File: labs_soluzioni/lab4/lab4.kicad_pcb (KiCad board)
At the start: 6 copper layers, 100 x 100 mm, 1 part, among them U1 XC7A35T-FGG484

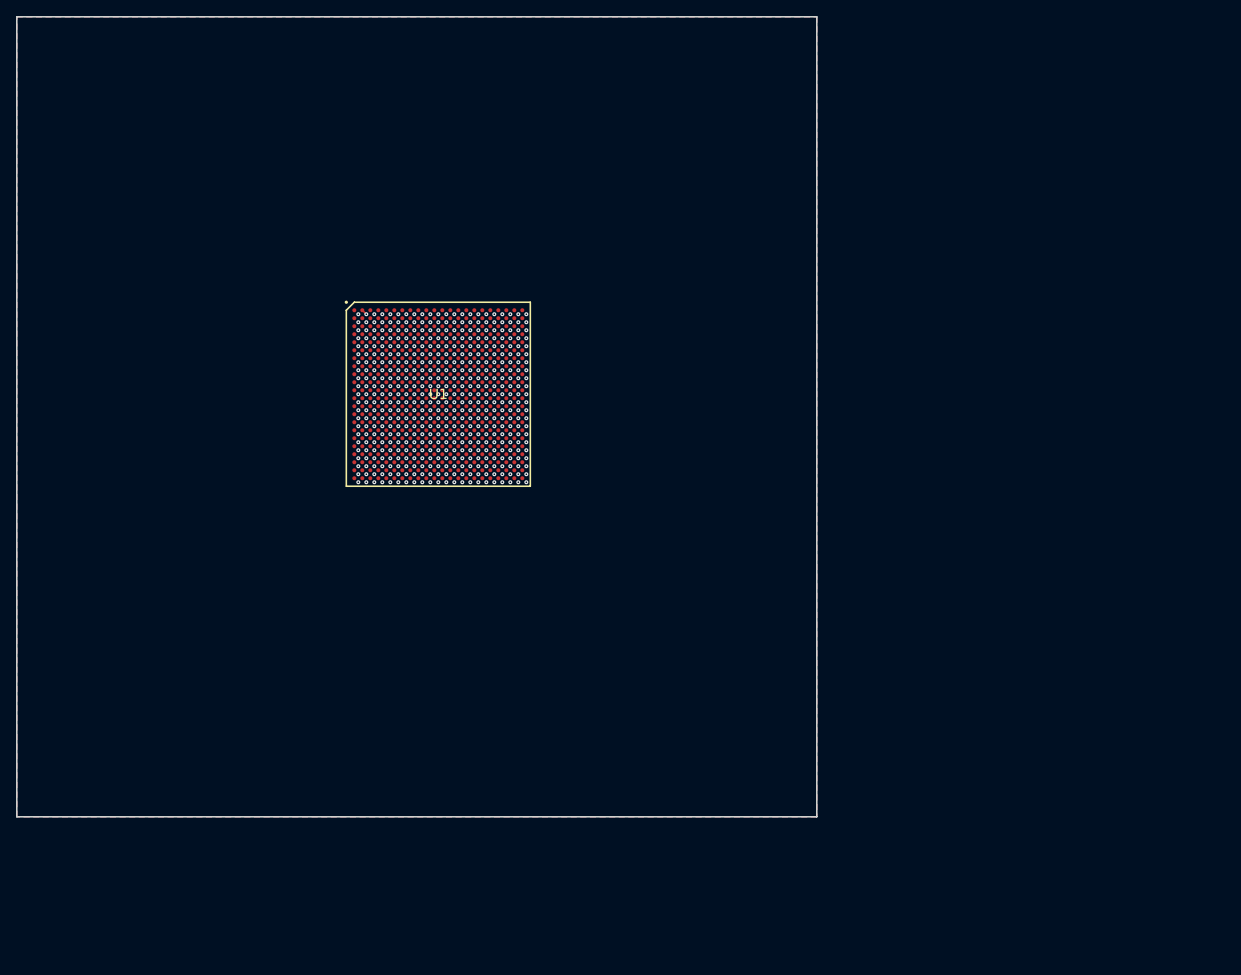
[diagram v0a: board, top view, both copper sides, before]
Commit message: NEW lab4
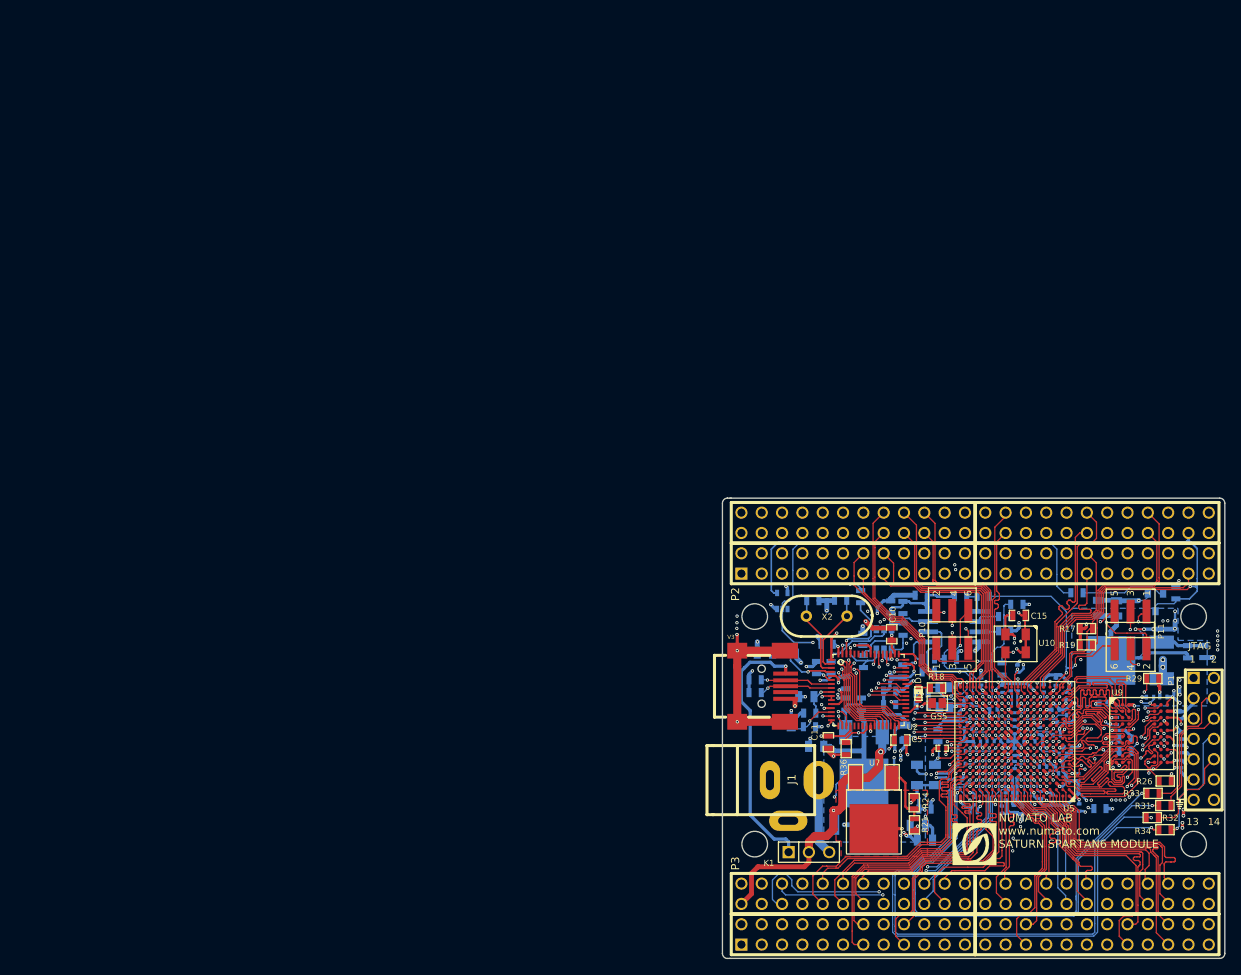
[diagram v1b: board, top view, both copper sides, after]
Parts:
- added 1PIN: P***, MH-3.2MM, F.Cu at (142.2, 125.0)
- added 1PIN: P***, MH-3.2MM, F.Cu at (197.1, 125.0)
- added 1PIN: P***, MH-3.2MM, F.Cu at (197.1, 153.4)
- added 1PIN: P***, MH-3.2MM, F.Cu at (142.2, 153.4)
- added C1: 0.1uF, SM0603_Capa, B.Cu at (151.3, 128.4)
- added C10: 0.1uF, SM0603_Capa, F.Cu at (159.4, 127.2)
- added C11: 0.1uF, SM0603_Capa, F.Cu at (151.5, 140.7)
- added C12: 0.1uF, SM0603_Capa, B.Cu at (155.8, 127.8)
- added C13: 0.1uF, SM0603_Capa, B.Cu at (146.7, 129.5)
- added C14: 0.1uF, SM0603_Capa, B.Cu at (149.1, 137.0)
- added C15: 0.1uF, SM0603_Capa, F.Cu at (175.3, 124.8)
- added C16: 15pF, SM0603_Capa, B.Cu at (165.1, 139.9)
- added C17: 0.01uF, SM0603_Capa, B.Cu at (159.1, 134.3)
- added C18: 0.01uF, SM0402_c, B.Cu at (177.9, 139.3)
- added C19: 0.01uF, SM0402_c, B.Cu at (180.7, 144.6)
- added C2: 0.1uF, SM0603_Capa, B.Cu at (153.6, 133.2)
- added C20: 0.01uF, SM0402_c, B.Cu at (174.7, 143.5)
- added C21: 0.01uF, SM0402_c, B.Cu at (173.6, 147.4)
- added C22: 0.01uF, SM0402_c, B.Cu at (174.7, 141.9)
- added C23: 0.01uF, SM0402_c, B.Cu at (169.6, 149.4)
- added C24: 0.01uF, SM0402_c, B.Cu at (178.3, 143.7)
- added C25: 0.01uF, SM0402_c, B.Cu at (179.5, 147.7)
- added C26: 0.01uF, SM0402_c, B.Cu at (174.7, 137.4)
- added C27: 0.01uF, SM0402_c, B.Cu at (169.8, 148.0)
- added C28: 0.01uF, SM0402_c, B.Cu at (172.1, 136.6)
- added C29: 0.01uF, SM0402_c, F.Cu at (165.7, 141.4)
- added C3: 0.1uF, SM0603_Capa, B.Cu at (160.7, 131.8)
- added C30: 0.01uF, SM0402_c, B.Cu at (174.7, 139.2)
- added C31: 0.01uF, SM0402_c, B.Cu at (170.5, 133.1)
- added C32: 0.01uF, SM0402_c, B.Cu at (173.4, 140.5)
- added C33: 0.01uF, SM0402_c, B.Cu at (175.1, 133.8)
- added C34: 0.01uF, SM0402_c, B.Cu at (177.7, 140.6)
- added C35: 0.01uF, SM0402_c, B.Cu at (174.2, 133.8)
- added C36: 0.01uF, SM0402_c, B.Cu at (171.7, 140.5)
- added C37: 0.01uF, SM0402_c, B.Cu at (168.1, 143.4)
- added C38: 0.01uF, SM0402_c, B.Cu at (175.4, 140.6)
- added C39: 0.01uF, SM0402_c, B.Cu at (179.8, 136.6)
- added C4: 0.1uF, SM0603_Capa, B.Cu at (159.1, 136.0)
- added C40: 0.01uF, SM0402_c, B.Cu at (178.4, 134.0)
- added C41: 0.01uF, SM0402_c, B.Cu at (168.9, 139.0)
- added C42: 0.01uF, SM0402_c, B.Cu at (182.8, 148.8)
- added C43: 0.01uF, SM0402_c, B.Cu at (180.5, 138.2)
- added C44: 0.01uF, SM0402_c, B.Cu at (175.7, 149.2)
- added C45: 0.01uF, SM0402_c, B.Cu at (181.4, 141.3)
- added C46: 0.01uF, SM0402_c, B.Cu at (174.7, 149.0)
- added C47: 0.01uF, SM0402_c, B.Cu at (180.3, 143.7)
- added C48: 0.01uF, SM0402_c, B.Cu at (175.1, 131.5)
- added C49: 0.01uF, SM0402_c, B.Cu at (181.1, 134.9)
- added C5: 0.1uF, SM0603_Capa, F.Cu at (160.4, 140.4)
- added C50: 0.01uF, SM0402_c, B.Cu at (167.8, 137.6)
- added C51: 0.01uF, SM0402_c, B.Cu at (182.7, 145.0)
- added C52: 0.01uF, SM0402_c, B.Cu at (173.2, 134.0)
- added C53: 0.01uF, SM0402_c, B.Cu at (191.7, 135.0)
- added C54: 0.01uF, SM0402_c, B.Cu at (181.7, 137.3)
- added C55: 0.01uF, SM0402_c, B.Cu at (168.1, 141.8)
- added C56: 0.01uF, SM0402_c, B.Cu at (179.9, 133.1)
- added C57: 0.01uF, SM0402_c, B.Cu at (167.7, 145.3)
- added C58: 0.01uF, SM0402_c, B.Cu at (180.0, 139.8)
- added C59: 0.01uF, SM0402_c, B.Cu at (173.1, 149.1)
- added C6: 22pF, SM0603_Capa, B.Cu at (153.0, 122.9)
- added C60: 0.01uF, SM0402_c, B.Cu at (178.0, 147.3)
- added C63: 0.01uF, SM0402_c, B.Cu at (170.0, 140.6)
- added C64: 0.01uF, SM0402_c, B.Cu at (168.8, 136.0)
- added C65: 47uF, SM1210, B.Cu at (153.7, 151.0)
- added C69: 10uF, SM0805, B.Cu at (185.2, 123.9)
- added C7: 0.1uF, SM0603_Capa, B.Cu at (163.5, 149.0)
- added C70: 10uF, SM0805, B.Cu at (149.9, 141.2)
- added C71: 10uF, SM0805, B.Cu at (162.6, 151.1)
- added C72: 0.1uF, SM0805, B.Cu at (187.5, 123.9)
- added C73: 0.1uF, SM0805, B.Cu at (161.0, 139.5)
- added C74: 0.1uF, SM0805, B.Cu at (163.5, 152.9)
- added C75: 0.1uF, SM0402_c, B.Cu at (185.8, 135.6)
- added C76: 0.1uF, SM0402_c, B.Cu at (180.8, 142.1)
- added C77: 0.1uF, SM0402_c, B.Cu at (195.5, 139.8)
- added C78: 0.1uF, SM0402_c, B.Cu at (195.5, 137.3)
- added C79: 0.1uF, SM0402_c, B.Cu at (195.5, 143.4)
- added C8: 0.1uF, SM0603_Capa, B.Cu at (163.1, 122.3)
- added C80: 0.1uF, SM0402_c, B.Cu at (193.3, 135.0)
- added C81: 0.1uF, SM0402_c, B.Cu at (195.5, 141.5)
- added C82: 0.1uF, SM0402_c, B.Cu at (187.5, 138.0)
- added C83: 15pF, SM0603_Capa, B.Cu at (173.1, 131.5)
- added C84: 0.01uF, SM0603_Capa, B.Cu at (159.2, 123.8)
- added C9: 22pF, SM0603_Capa, B.Cu at (149.5, 123.0)
- added D1: LED, LED-0603, F.Cu at (162.7, 134.6)
- added G***: LOGO, LOGO, F.Cu at (169.7, 153.4)
- added GS5: GS2, GS2, F.Cu at (165.1, 135.8)
- added GS6: GS2, GS2, B.Cu at (165.9, 133.8)
- added GS7: GS2, GS2, B.Cu at (166.0, 136.3)
- added J1: JACK_2P, JACK_ALIM, F.Cu at (144.1, 145.4)
- added K1: CONN_3, PIN_ARRAY_3X1, F.Cu at (149.0, 154.4)
- added L1: INDUCTOR, SM0805, B.Cu at (143.5, 129.5)
- added L2: INDUCTOR, SM0805, B.Cu at (148.7, 135.0)
- added P1: CONN_7X2, pin_array_7x2, F.Cu at (198.4, 141.5)
- added P10: CONN_3X2, pin_array_2mm_3x2_SMD, F.Cu at (166.9, 126.6)
- added P11: CONN_3X2, pin_array_2mm_3x2_SMD, F.Cu at (189.2, 126.6)
- added P2: CONN_12X2, pin_array_12x2, F.Cu at (154.6, 159.6)
- added P3: CONN_12X2, pin_array_12x2, F.Cu at (154.6, 164.7)
- added P4: CONN_12X2, pin_array_12x2, F.Cu at (185.0, 159.6)
- added P5: CONN_12X2, pin_array_12x2, F.Cu at (185.0, 164.7)
- added P6: CONN_12X2, pin_array_12x2, F.Cu at (154.6, 118.3)
- added P7: CONN_12X2, pin_array_12x2, F.Cu at (154.6, 113.2)
- added P8: CONN_12X2, pin_array_12x2, F.Cu at (185.0, 113.2)
- added P9: CONN_12X2, pin_array_12x2, F.Cu at (185.0, 118.3)
- added Q1: NPN, SOT23, B.Cu at (192.3, 123.2)
- added R1: 10K, SM0603, B.Cu at (160.8, 126.5)
- added R10: 10K, SM0603, B.Cu at (173.5, 126.7)
- added R11: 10K, SM0603, B.Cu at (168.0, 122.5)
- added R12: 0R, SM0603, B.Cu at (163.9, 130.3)
- added R13: 10K, SM0603, B.Cu at (160.8, 123.8)
- added R14: 4.7K, SM0603, B.Cu at (185.4, 149.0)
- added R15: 10K, SM0603, B.Cu at (163.2, 136.0)
- added R16: 10K, SM0603, B.Cu at (163.2, 134.5)
- added R17: 4.7K, SM0603, F.Cu at (183.7, 126.5)
- added R18: 1K, SM0603, F.Cu at (165.0, 133.9)
- added R19: 4.7K, SM0603, F.Cu at (183.7, 128.5)
- added R2: 2K2, SM0603, B.Cu at (155.8, 130.6)
- added R20: 330R, SM0603, B.Cu at (153.6, 135.9)
- added R21: 0R, SM0603, F.Cu at (162.2, 151.0)
- added R22: 100R, SM0603, B.Cu at (198.4, 129.3)
- added R23: 220R, SM0603, B.Cu at (155.6, 135.9)
- added R24: 220R, SM0603, F.Cu at (162.2, 148.2)
- added R25: 220R, SM0603, B.Cu at (196.3, 129.4)
- added R26: 100R, SM0603, F.Cu at (193.6, 145.5)
- added R27: 100R, SM0603, B.Cu at (188.6, 141.8)
- added R28: 4.7K, SM0603, B.Cu at (188.5, 140.3)
- added R29: 100R, SM0603, F.Cu at (192.0, 132.7)
- added R3: 10K, SM0603, B.Cu at (175.0, 123.4)
- added R30: 10K, SM0603, B.Cu at (166.7, 130.3)
- added R31: 0R, SM0603, F.Cu at (193.5, 148.6)
- added R32: 0R, SM0603, F.Cu at (191.9, 150.1)
- added R33: 0R, SM0603, F.Cu at (192.0, 147.1)
- added R34: 0R, SM0603, F.Cu at (193.5, 151.6)
- added R35: 10K, SM0603, B.Cu at (182.5, 122.0)
- added R36: 10K, SM0603, F.Cu at (153.7, 141.5)
- added R37: 10K, SM0603, B.Cu at (151.8, 131.4)
- added R38: 10K, SM0603, B.Cu at (155.5, 122.5)
- added R39: 2.2K, SM0603, B.Cu at (194.9, 122.0)
- added R4: 0R, SM0603, B.Cu at (163.9, 131.9)
- added R5: 12K, SM0603, B.Cu at (150.0, 131.3)
- added R6: 4K7, SM0603, B.Cu at (149.1, 138.7)
- added R7: 10K, SM0603, B.Cu at (146.8, 138.2)
- added R8: 0R, SM0603, B.Cu at (170.8, 122.4)
- added R9: 0R, SM0603, B.Cu at (173.5, 125.0)
- added U10: FXO-HC536R, FXO-HC536R, F.Cu at (174.8, 128.3)
- added U11: 74LVC1GU04, sot323-5, B.Cu at (145.7, 123.0)
- added U2: FT2232H, QFN64, F.Cu at (156.5, 134.2)
- added U3: M25P16, SO8E_N, B.Cu at (167.1, 126.2)
- added U4: FXO-HC536R, FXO-HC536R, B.Cu at (163.6, 144.8)
- added U5: SPARTAN6LXXXX-CSG324, CSG324, F.Cu at (174.8, 140.6)
- added U6: LM1117, DPAK2, B.Cu at (155.9, 139.4)
- added U7: LM1117, DPAK2, F.Cu at (157.1, 145.1)
- added U8: LM1117, DPAK2, B.Cu at (193.1, 130.5)
- added U9: MT46H32M16LF, BGA60, F.Cu at (190.6, 139.6)
- added VR1: VR, SM0603, B.Cu at (142.3, 132.9)
- added VR2: VR, SM0603, B.Cu at (142.3, 134.5)
- added X1: USBMINI, USBMICRO, F.Cu at (143.1, 133.7)
- added X2: CRYSTAL, HC-49V, F.Cu at (151.2, 124.9)
- U1: value XC7A35T-FGG484 -> 93LC46; footprint Package_BGA:BGA484C100P22X22_2300X2300X260 -> SOT23_6; moved to B.Cu
- moved U1 63.6 mm to (158.4, 127.8), turned to 180 degrees
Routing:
- net GND: track 0.71 -> 301.1 mm, vias 1 -> 121
- net VCC3V3: track 0.00 -> 226.4 mm, vias 0 -> 57
- net VCCIN: track 0.00 -> 131.9 mm, vias 0 -> 4
- net /FTDI2232H/PROGB: track 0.00 -> 105.8 mm, vias 0 -> 1
- net /FTDI2232H/TDI: track 0.00 -> 76.8 mm, vias 0 -> 3
- net /FTDI2232H/TDO: track 0.00 -> 76.5 mm, vias 0 -> 4
- net N-0000045: track 0.00 -> 74.5 mm, vias 0 -> 2
- net DDR1V8: track 0.00 -> 73.5 mm, vias 0 -> 31
- net N-0000074: track 0.00 -> 71.4 mm, vias 0 -> 2
- net N-0000075: track 0.00 -> 71.3 mm, vias 0 -> 2
- net N-0000073: track 0.00 -> 61.8 mm, vias 0 -> 2
- net /FTDI2232H/TCK/SCK: track 0.00 -> 58.2 mm, vias 0 -> 3
- net N-0000080: track 0.00 -> 57.9 mm, vias 0 -> 2
- net /GPIOS/GPIO-P13: track 0.00 -> 51.5 mm, vias 0 -> 1
- net /GPIOS/GPIO-N13: track 0.00 -> 51.5 mm, vias 0 -> 1
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- added copper zone on B.Cu, net DDR1V8
- added copper zone on In4.Cu, net DDR1V8
- added copper zone on In1.Cu, net GND
- added copper zone on F.Cu, net VCC1V2
- added copper zone on In4.Cu, net VCC1V2
- added copper zone on B.Cu, net VCC3V3
- added copper zone on In4.Cu, net VCC3V3
- removed copper zone on B.Cu, net (none)
- removed copper zone on F.Cu, net (none)
- removed copper zone on In1.Cu, net (none)
- removed copper zone on In4.Cu, net (none)
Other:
- board size 100 x 100 mm -> 62.8 x 57.5 mm
- rule pad_to_mask_clearance: 0 -> 0.254
- board text added: "1"
- board text added: "1 2 3"
- board text added: "1-2 EXT PWR 2-3 USB PWR"
- board text added: "13"
- board text added: "14"
- board text added: "2"
- board text added: "3"
- board text added: "4"
- board text added: "5"
- board text added: "6"
- board text added: "93"
- board text added: "96"
- board text added: "JTAG"
- board text added: "NUMATO LAB www.numato.com SATURN SPARTAN6 MODULE"
- board text added: "P2"
- board text added: "P3"
- board text added: "V3"
